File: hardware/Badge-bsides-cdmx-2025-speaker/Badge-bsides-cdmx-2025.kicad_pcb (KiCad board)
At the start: 2 copper layers, 50 x 110 mm, 30 parts, among them J1 SWDIO, J3 ADDON, J4 Conn_01x04_Pin, J5 I2C, J6 Conn_01x04_Pin, P6 USB_C_Plug_USB2.0, Q3 DMG3415U-7, SW11 ON, SW2 RESET, U1 PY32F030F28U6TR, U6 AP2112K-3.3

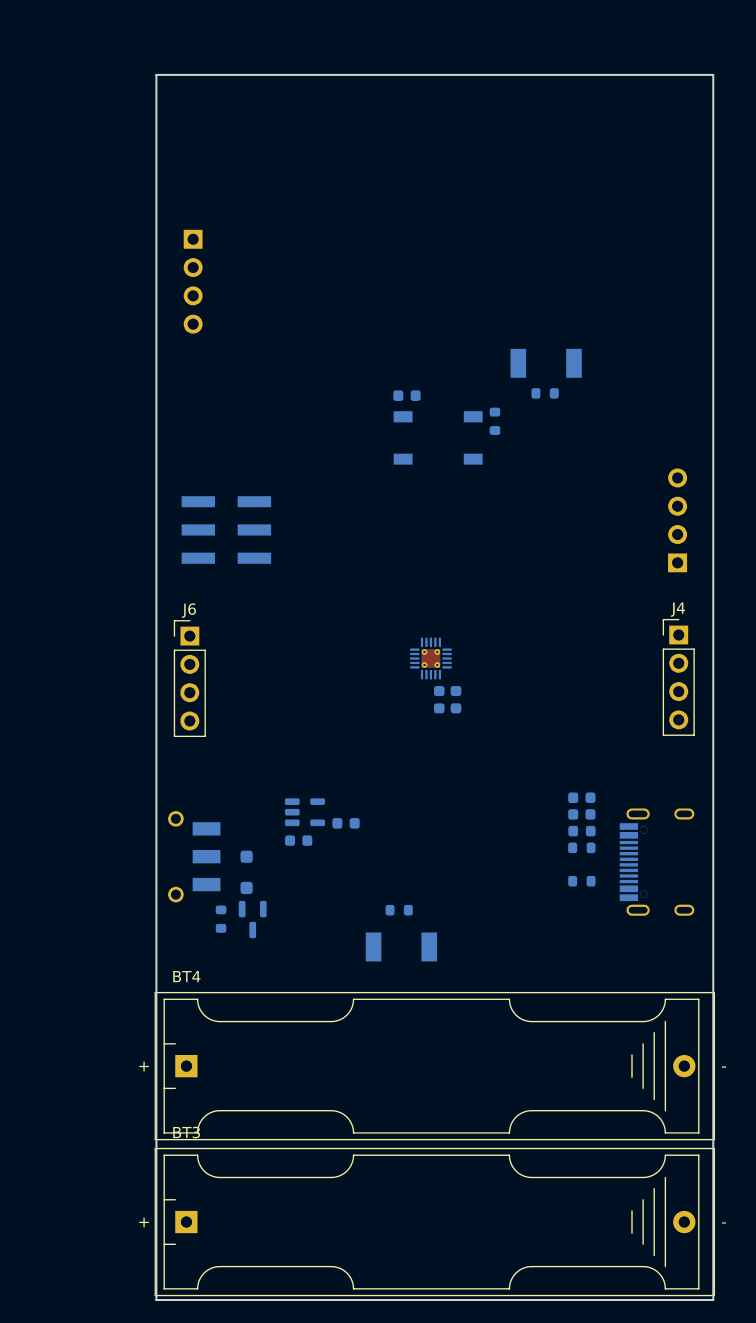
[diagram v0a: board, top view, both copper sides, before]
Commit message: feat(Hw):started_routing
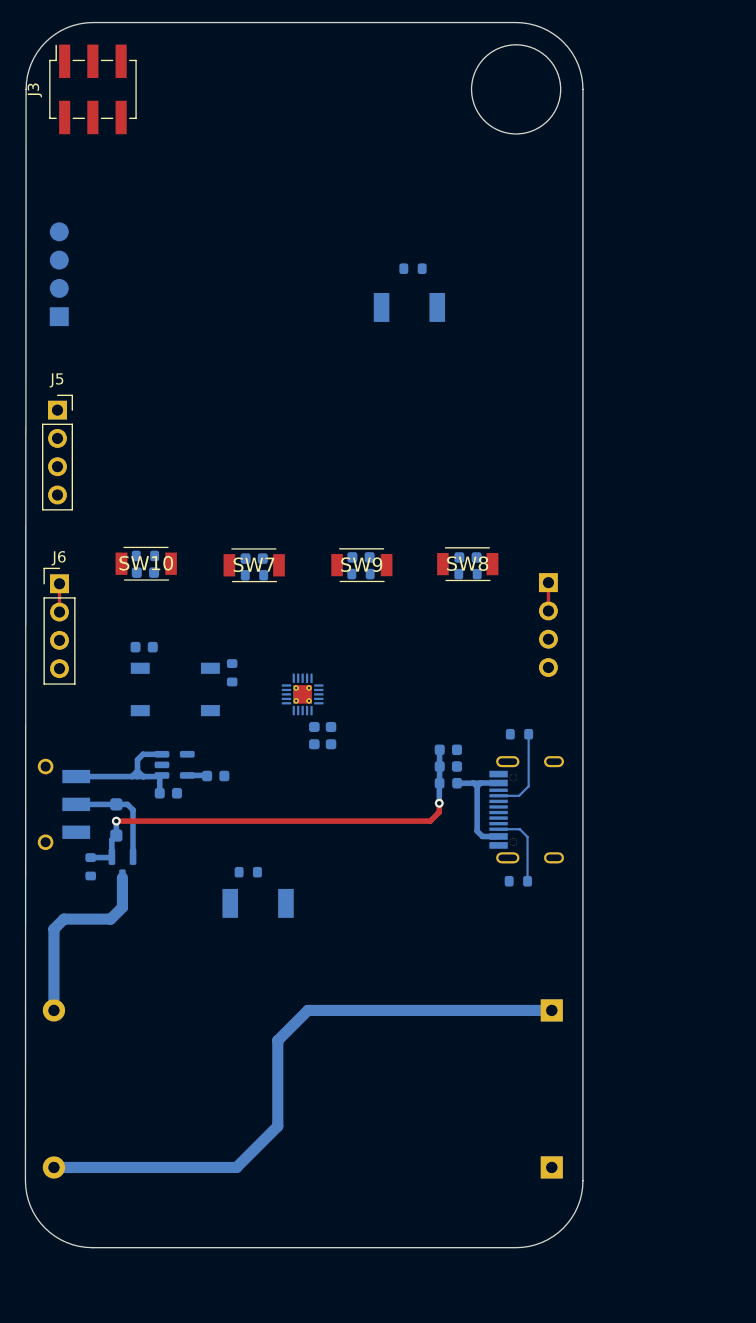
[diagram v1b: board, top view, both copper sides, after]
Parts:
- added C67: 10uF, Capacitor_SMD:C_0603_1608Metric, B.Cu at (153.0, 82.3)
- added C68: 10uF, Capacitor_SMD:C_0603_1608Metric, B.Cu at (143.4, 82.3)
- added C69: 10uF, Capacitor_SMD:C_0603_1608Metric, B.Cu at (133.8, 82.4)
- added C70: 10uF, Capacitor_SMD:C_0603_1608Metric, B.Cu at (124.0, 83.7)
- added R5: 10k, Resistor_SMD:R_0603_1608Metric, B.Cu at (153.0, 83.8)
- added R6: 10k, Resistor_SMD:R_0603_1608Metric, B.Cu at (143.4, 83.8)
- added R7: 10k, Resistor_SMD:R_0603_1608Metric, B.Cu at (133.8, 83.9)
- added R8: 10k, Resistor_SMD:R_0603_1608Metric, B.Cu at (124.0, 82.2)
- added SW10: SW_Push, Footprints:TS1088R02026, F.Cu at (124.1, 82.9)
- added SW7: SW_Push, Footprints:TS1088R02026, F.Cu at (133.8, 83.0)
- added SW8: SW_Push, Footprints:TS1088R02026, F.Cu at (152.9, 82.9)
- added SW9: SW_Push, Footprints:TS1088R02026, F.Cu at (143.4, 83.0)
- BT3, BT4, J4: moved to B.Cu
- J3, J5: moved to F.Cu
- moved J1 59.8 mm to (116.3, 60.7)
- moved J3 41.3 mm to (119.3, 40.3), turned to 90 degrees
- moved BT3 37.9 mm to (160.5, 123.0), turned to 180 degrees
- moved BT4 34.0 mm to (160.5, 137.1), turned to 180 degrees
- moved SW2 32.7 mm to (126.7, 94.2)
- moved R4 32.7 mm to (131.8, 92.7)
- moved C6 32.7 mm to (123.9, 90.4)
- moved J5 19.6 mm to (116.1, 69.1), turned to 0 degrees
- moved R11 16.3 mm to (148.0, 56.4), turned to 180 degrees
- moved R9 14.0 mm to (133.2, 110.6), turned to 0 degrees
- moved D9 13.5 mm to (134.1, 113.4), turned to 0 degrees
- moved C33 13.3 mm to (151.2, 99.6)
- moved D10 13.3 mm to (147.7, 59.9)
- moved F3 12.7 mm to (151.2, 102.6)
- moved J4 12.6 mm to (160.2, 84.6), turned to 180 degrees
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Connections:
- BT3 pad 2: +3.3V -> +BATT
- J3 pad 5: /GPIO1 -> /GPIO2
- J3 pad 6: /GPIO2 -> /GPIO1
- U1 pad 1: unconnected-(U1-PA5-Pad1) -> /BTTN2
- U1 pad 10: unconnected-(U1-PB6-Pad10) -> /LED1
- U1 pad 16: /GPIO2 -> /BTTN4
- U1 pad 17: /GPIO1 -> /BTTN3
- U1 pad 2: /LED1 -> /BTTN1
- U1 pad 20: unconnected-(U1-PA4-Pad20) -> /LED2
- U1 pad 3: /LED2 -> /GPIO1
- U1 pad 5: unconnected-(U1-PA12-Pad5) -> /GPIO2
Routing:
- net Net-(BT3--): track 0.00 -> 55.1 mm
- net VBUS: track 0.00 -> 40.2 mm, vias 0 -> 2
- net +BATT: track 0.00 -> 16.9 mm
- net Net-(SW11-A): track 0.00 -> 14.8 mm
- net Net-(F3-Pad1): track 0.00 -> 10.8 mm
- net Net-(D4-K): track 0.00 -> 9.51 mm
- net Net-(P6-CC): track 0.00 -> 7.73 mm
- net Net-(P6-VCONN): track 0.00 -> 6.86 mm
- net /TX: track 0.00 -> 2.54 mm
- net /RX: track 0.00 -> 2.54 mm
- net +3V3: track 0.00 -> 1.80 mm
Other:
- board size 50 x 110 mm -> 50.1 x 110 mm
